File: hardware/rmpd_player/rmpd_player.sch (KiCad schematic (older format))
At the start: 14 parts

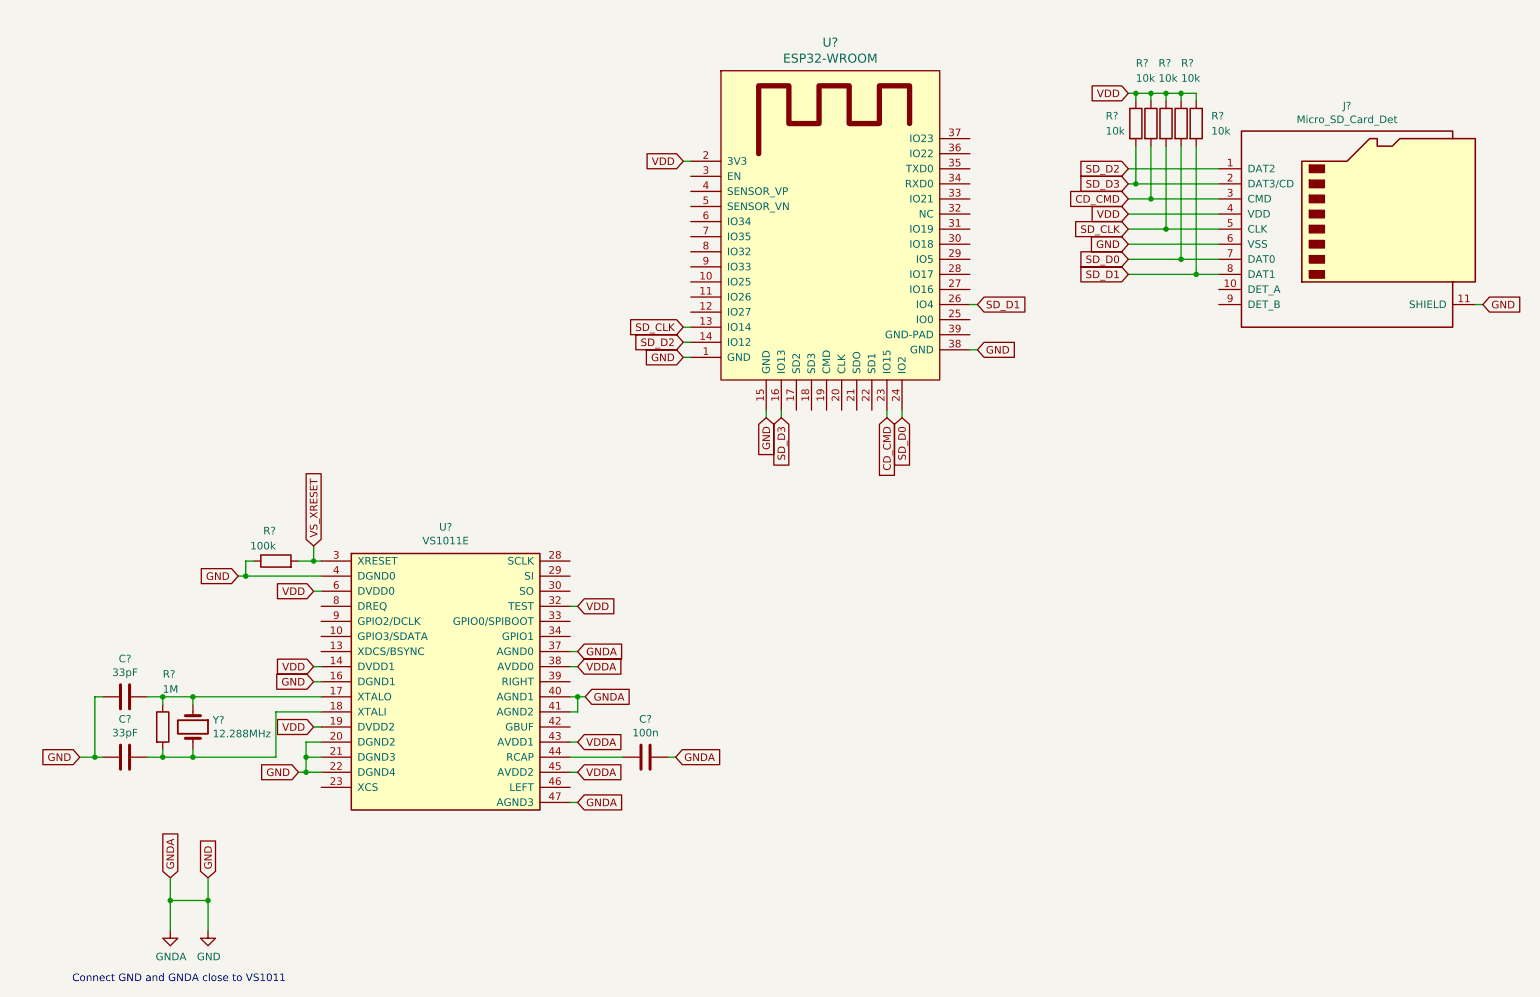
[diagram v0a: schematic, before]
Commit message: more schematic
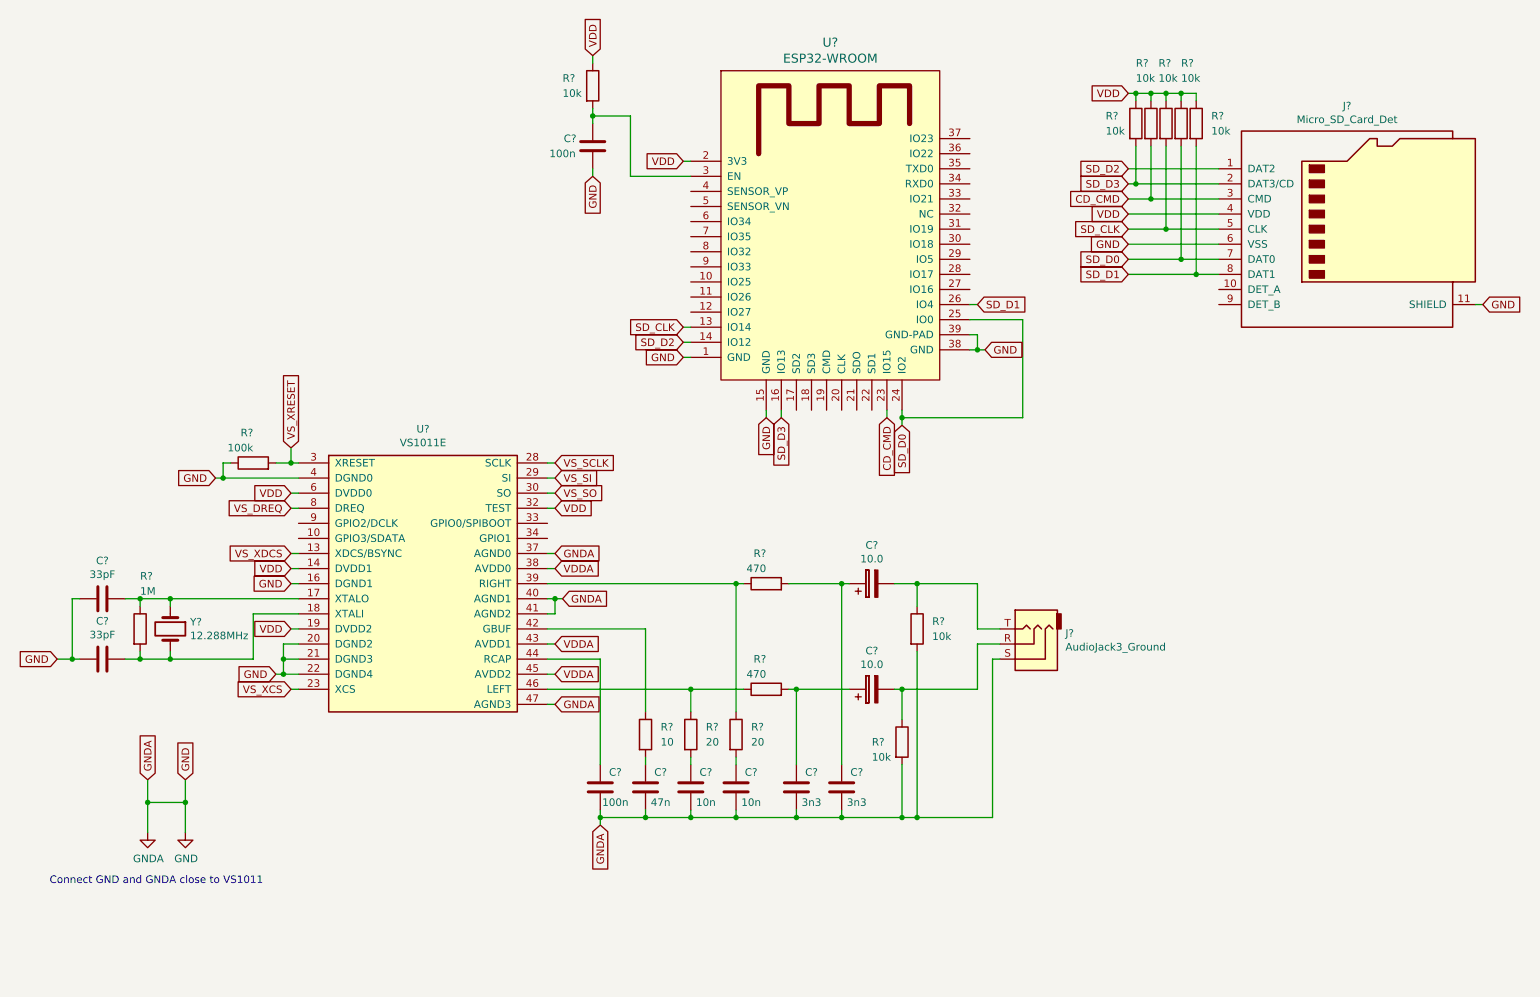
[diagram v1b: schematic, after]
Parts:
- added C?: 100n, symbol Device:C
- added C?: 47n, symbol Device:C
- added C? (x2): 10n, symbol Device:C
- added C? (x2): 3n3, symbol Device:C
- added C? (x2): 10.0, symbol Device:CP
- added J?: AudioJack3_Ground, symbol Connector:AudioJack3_Ground
- added R? (x3): 10k, symbol Device:R
- added R?: 10, symbol Device:R
- added R? (x2): 20, symbol Device:R
- added R? (x2): 470, symbol Device:R
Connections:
- net GND: now also C?.2, U?.39 (GND-PAD), C?.1, C?.1, C?.1, C?.1, C?.1, C?.1, J?.S, R?.2, R?.2; no longer C?.1
- net SD_D0: now also U?.25 (IO0)
- net VDD: now also R?.1
- net at U?.3 (EN): now also C?.2, R?.2
- net VS_XDCS: now reaches U?.13 (XDCS/BSYNC)
- net VS_XCS: now reaches U?.23 (XCS)
- net VS_SCLK: now reaches U?.28 (SCLK)
- net VS_SI: now reaches U?.29 (SI)
- net VS_SO: now reaches U?.30 (SO)
- net at U?.39 (RIGHT): now also R?.1, R?.1
- net at U?.42 (GBUF): now also R?.1
- net at U?.44 (RCAP): now also C?.1; no longer C?.2
- net at U?.46 (LEFT): now also R?.1, R?.1
- net VS_DREQ: now reaches U?.8 (DREQ)
- new net: C?.2, R?.2 (x3)
- new net: C?.1, C?.2, R?.2 (x2)
- new net: C?.2, J?.T, R?.1
- new net: C?.2, J?.R, R?.1
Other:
- moved on the sheet: C?, R?, U?, Y?
